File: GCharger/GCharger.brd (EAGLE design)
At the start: 160 x 100 mm, 0 parts

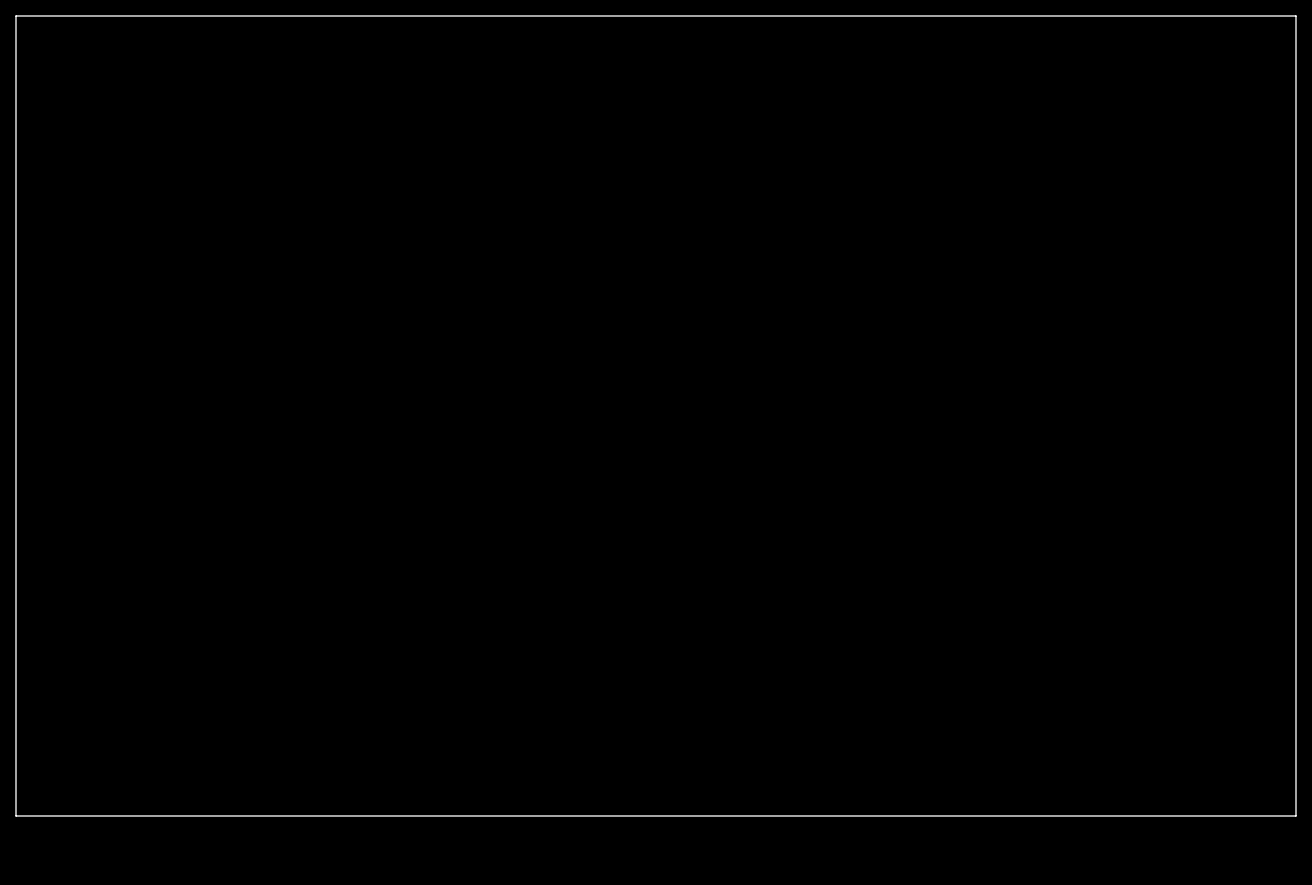
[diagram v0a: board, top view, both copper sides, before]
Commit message: Gcharger Board
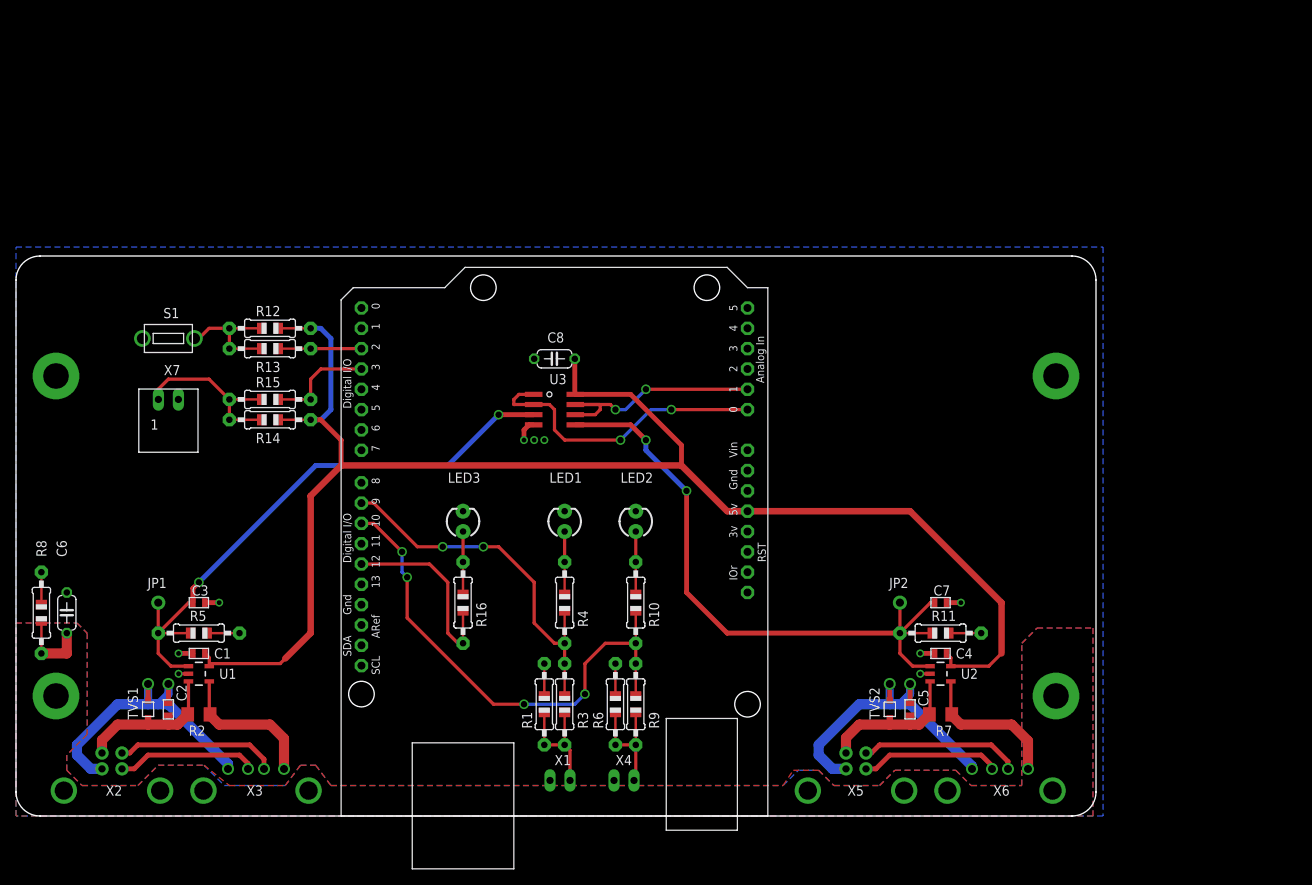
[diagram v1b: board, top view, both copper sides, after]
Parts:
- added C1, C2, C4, C5: (no value), Gcharger:C0603(1608)
- added C3, C7: DNP, g-project:C0603(1608)
- added C6, C8: 0.1uF monolithic, adafruit:C050-024X044
- added H1, H2, H3, H4: MOUNT-PAD-ROUND3.2, OSSI:3.2-PAD-ROUND
- added JP1, JP2: (no value), adafruit:1X01-CLEANBIG
- added LED1, LED2: Red, SparkFun-LED:LED3MM
- added LED3: Green, SparkFun-LED:LED3MM
- added R1, R12, R14, R6: 47k, g-project:0805-THM
- added R10, R16, R4: 1.5k, g-project:0805-THM
- added R11, R5: 10k, 1%, g-project:0805-THM
- added R13, R15, R3, R9: 4.7k, g-project:0805-THM
- added R2, R7: 0.1, 1% Current Sense, SparkFun-Resistors:1206
- added R8: 510, g-project:0805-THM
- added S1: (no value), WaterDrop:SKHLACA010
- added TVS1, TVS2: SD0, Gcharger:SOD-323
- added U1, U2: INA169, Gcharger:SOT23-5
- added U3: TLV2462, Gcharger:SO8
- added U4: ARDUINOR3-TPLACE, Gcharger:ARDUINOR3
- added X1, X4, X7: 5268-02, OSSI:5628-02
- added X2, X5: USB-B, Gcharger:USB-B-PTH
- added X3, X6: USB-A-Recep, Gcharger:USB-A-RECEPT
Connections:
- new net +5V: C1.2, C4.2, C8.1, R12.2, R14.2, U1.5, U2.5, U3.8, U4.5V
- new net +5V_USB_1: C2.2, R2.1, TVS1.1, U1.3, X2.VBUS
- new net +5V_USB_2: C5.2, R7.1, TVS2.1, U2.3, X5.VBUS
- new net 3V: U4.3V
- new net CURRENT1: C3.1, JP1.1, R5.2, U1.1, U3.3
- new net CURRENT2: C7.1, JP2.1, R11.2, U2.1, U3.5
- new net GND: C1.1, C3.2, C4.1, C6.2, C7.2, C8.2, LED1.K, LED2.K, LED3.K, R1.2, R11.1, R5.1, R6.2, R8.2, S1.P$1, U1.2, U2.2, U3.4, U4.GND, U4.GND1, U4.GND2, X1.2, X4.2, X7.2
- new net I_ADC1: U3.1, U3.2, U4.A0
- new net I_ADC2: U3.6, U3.7, U4.A1
- new net I_GND1: C2.1, TVS1.2, X2.GND, X3.4
- new net I_GND2: C5.1, TVS2.2, X5.GND, X6.4
- new net LED1: R16.2, U4.D12
- new net N$1: X5.D-, X6.2
- new net N$10: LED2.A, R10.1
- new net N$11: LED1.A, R4.1
- new net N$12: LED3.A, R16.1
- new net N$13: R14.1, R15.1, X7.1
- new net N$2: X5.D+, X6.3
- new net N$3: R1.1, R3.2, X1.1
- new net N$4: X2.D-, X3.2
- new net N$5: X2.D+, X3.3
- new net N$6: R7.2, U2.4, X6.1
- new net N$7: R12.1, R13.1, S1.P$2
- new net N$8: R6.1, R9.2, X4.1
- new net N$9: R2.2, U1.4, X3.1
- new net OUT1: R3.1, R4.2, U4.D9
- new net OUT2: R10.2, R9.1, U4.D10
- new net STRUT_GND: C6.1, H1.B3,2, R8.1, X2.S1, X2.S2, X3.S1, X3.S2, X5.S1, X5.S2, X6.S1, X6.S2
- new net SW1: R13.2, U4.D2
- new net SW2: R15.2, U4.D3
- new net VIN: U4.VIN
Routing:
- net +5V: track 0.00 -> 189.5 mm
- net CURRENT2: track 0.00 -> 76.2 mm, vias 0 -> 2
- net CURRENT1: track 0.00 -> 70.1 mm, vias 0 -> 2
- net OUT2: track 0.00 -> 56.0 mm, vias 0 -> 4
- net I_GND2: track 0.00 -> 40.3 mm, vias 0 -> 2
- net I_GND1: track 0.00 -> 39.9 mm, vias 0 -> 2
- net OUT1: track 0.00 -> 38.2 mm, vias 0 -> 2
- net I_ADC1: track 0.00 -> 37.5 mm, vias 0 -> 2
- net I_ADC2: track 0.00 -> 30.0 mm, vias 0 -> 2
- net LED1: track 0.00 -> 20.5 mm
- net N$4: track 0.00 -> 20.1 mm
- net N$1: track 0.00 -> 20.0 mm
- net +5V_USB_1: track 0.00 -> 19.8 mm
- net +5V_USB_2: track 0.00 -> 19.6 mm
- net N$6: track 0.00 -> 18.7 mm
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- added copper zone on layer 16, net GND
- added copper zone on layer 1, net STRUT_GND
- added copper zone on layer 16, net STRUT_GND
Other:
- board size 160 x 100 mm -> 135 x 70 mm
